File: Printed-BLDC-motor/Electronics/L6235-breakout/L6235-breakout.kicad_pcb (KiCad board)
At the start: 2 copper layers, 56.9 x 39.2 mm, 30 parts, among them J1 CONTROL, J2 HALL, J3 MOTOR, J4 5V, J5 PWR, U1 L6235PD

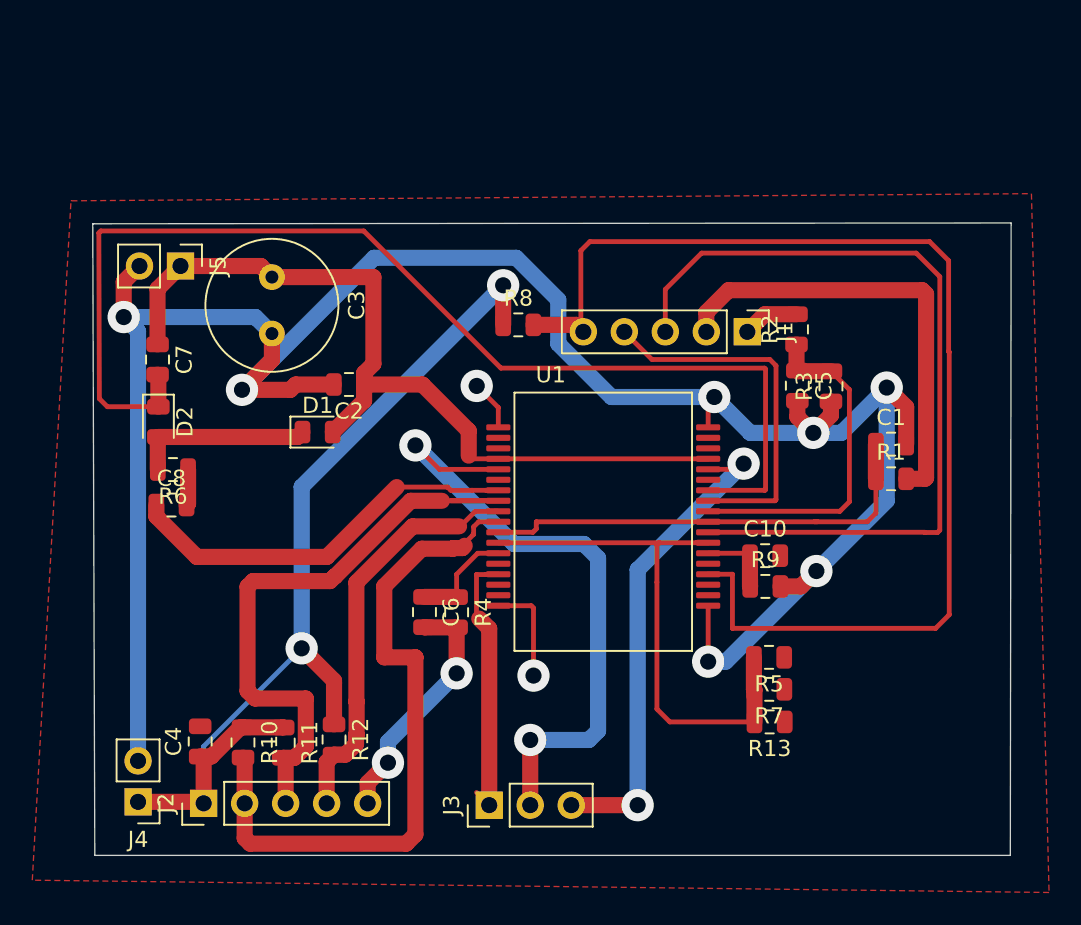
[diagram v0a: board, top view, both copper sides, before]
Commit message: Latest BLDC driver PCB.
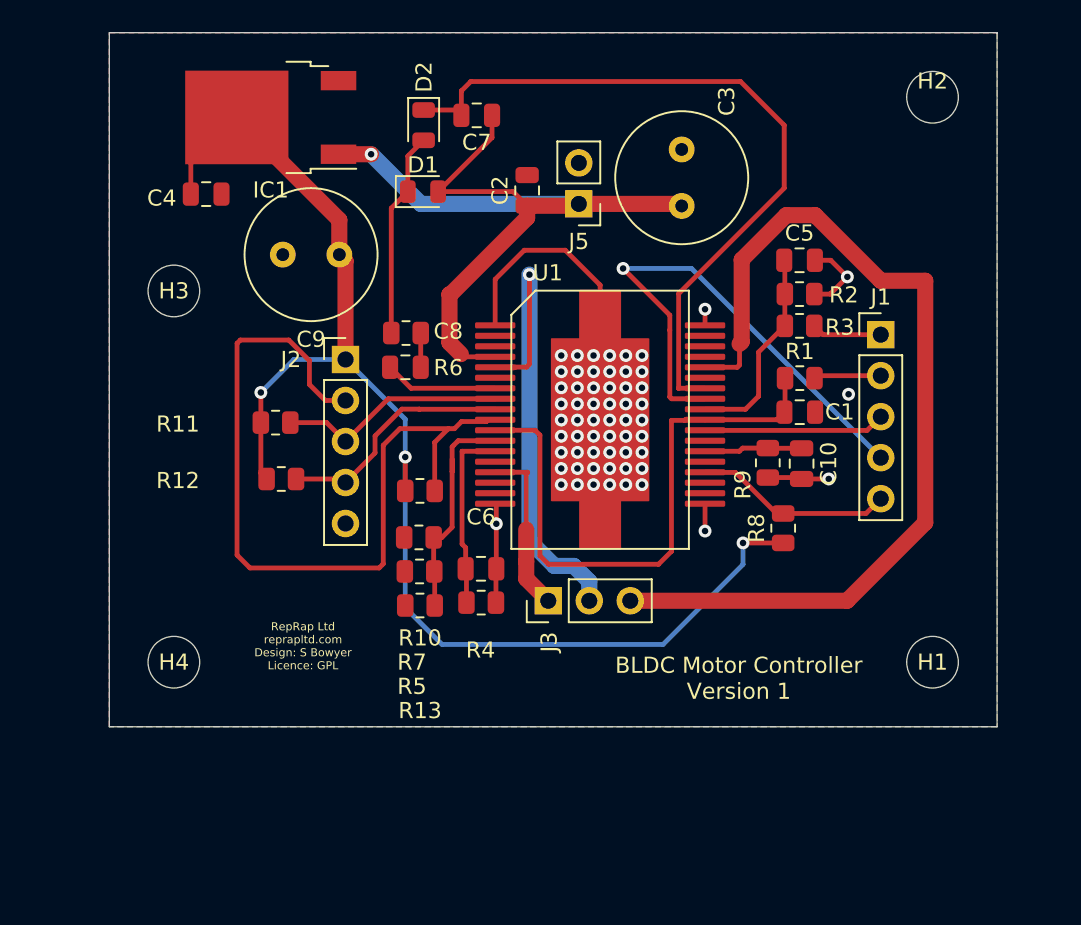
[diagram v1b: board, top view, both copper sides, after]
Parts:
- removed J4: 5V, Connector_PinHeader_2.54mm:PinHeader_1x02_P2.54mm_Vertical
- added C9: 100u, Capacitor_THT:C_Radial_D8.0mm_H7.0mm_P3.50mm, F.Cu at (15.2, 160.8)
- added H1: MountingHole, MountingHole:MountingHole_3.2mm_M3, F.Cu at (52.0, 186.0)
- added H2: MountingHole, MountingHole:MountingHole_3.2mm_M3, F.Cu at (52.0, 151.0)
- added H3: MountingHole, MountingHole:MountingHole_3.2mm_M3, F.Cu at (5.00, 163.0)
- added H4: MountingHole, MountingHole:MountingHole_3.2mm_M3, F.Cu at (5.00, 186.0)
- added IC1: 7805DT, Package_TO_SOT_SMD:TO-252-2, F.Cu at (11.0, 152.2)
- moved C4 33.9 mm to (7.00, 157.0), turned to 0 degrees
- moved J2 28.9 mm to (15.6, 167.2), turned to 0 degrees
- moved C3 25.8 mm to (36.5, 157.7), turned to 90 degrees
- moved J5 25.0 mm to (30.1, 157.6), turned to 180 degrees
- moved C7 24.9 mm to (23.8, 152.1), turned to 180 degrees
- moved D2 24.7 mm to (20.5, 152.7)
- moved R7 23.7 mm to (20.2, 178.3), turned to 0 degrees
- moved R13 22.8 mm to (20.2, 182.5), turned to 0 degrees
- moved R5 22.3 mm to (20.2, 180.4), turned to 0 degrees
- moved R8 20.7 mm to (42.7, 177.7), turned to 90 degrees
- moved R11 19.8 mm to (11.3, 171.2), turned to 0 degrees
- moved R10 19.1 mm to (20.2, 175.4), turned to 0 degrees
- moved C8 16.8 mm to (19.3, 167.7)
- moved R6 16.7 mm to (19.4, 165.6)
- moved R12 16.5 mm to (11.7, 174.7), turned to 0 degrees
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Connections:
- U1 pad 25: Net-(R13-Pad2) -> Net-(U1-Pad25)
- U1 pad 33: VSS -> Net-(U1-Pad33)
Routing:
- net GND: track 165.5 -> 36.9 mm, vias 11 -> 60
- net TACHO: track 72.5 -> 12.3 mm
- net F-R: track 51.3 -> 11.2 mm
- net PHASE3: track 30.3 -> 58.2 mm, vias 2 -> 0
- net Net-(C7-Pad2): track 72.1 -> 46.0 mm
- net Net-(J1-Pad2): track 28.1 -> 4.17 mm
- net HALL2: track 37.8 -> 14.3 mm
- net +5V: track 60.8 -> 82.4 mm, vias 2 -> 3
- net Net-(R13-Pad2): track 34.5 -> 14.2 mm
- net Net-(C8-Pad1): track 25.6 -> 7.05 mm
- net HALL3: track 25.5 -> 14.9 mm
- net BRAKE: track 22.8 -> 32.2 mm, vias 0 -> 1
- net PHASE2: track 39.1 -> 30.2 mm, vias 2 -> 1
- net VREF: track 21.3 -> 12.8 mm
- net HALL1: track 42.6 -> 51.0 mm
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- added copper zone on B.Cu, net GND
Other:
- board size 56.9 x 39.2 mm -> 55 x 43 mm
- board text added: "BLDC Motor Controller Version 1"
- board text added: "RepRap Ltd reprapltd.com Design: S Bowyer Licence: GPL"
